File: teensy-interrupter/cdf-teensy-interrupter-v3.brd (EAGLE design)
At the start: 66 x 45.7 mm, 42 parts, among them IC1 TP4056, Q1 BC817-40LT1SMD

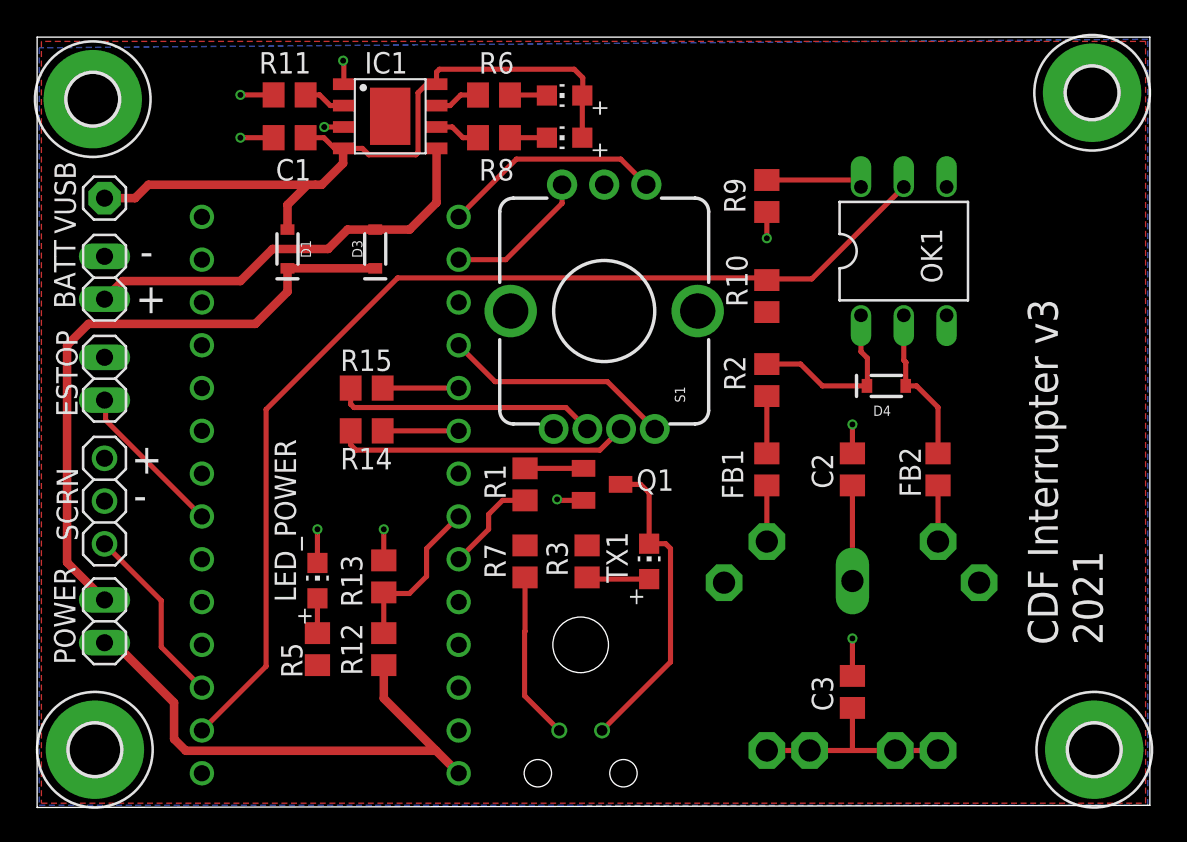
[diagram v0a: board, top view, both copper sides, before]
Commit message: V3r1
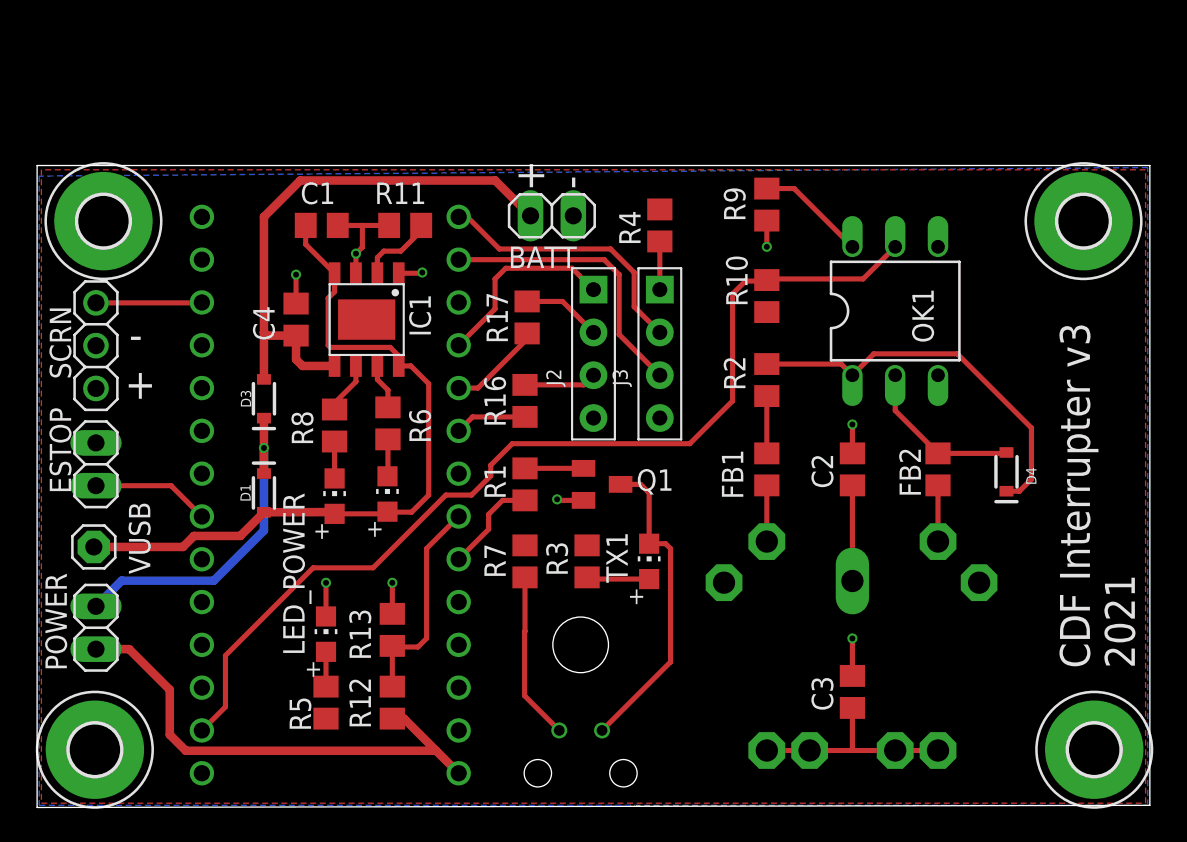
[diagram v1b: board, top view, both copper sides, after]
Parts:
- removed R14, R15: 100, rcl:R0805
- removed S1: ENCODER-2LED, SparkFun-Switches:ENCODER_LED_2
- added C4: 10uF, rcl:C0805
- added J2, J3: 4p-2.54, OPL_Connector:H4-2.54
- added R16, R17: 100, rcl:R0805
- added R4: 10k, rcl:R0805
- R11: value 1.2K -> 10k
- moved BATT 26.8 mm to (30.6, 35.1), turned to 180 degrees
- moved CHARGING 25.9 mm to (20.8, 18.6), turned to 0 degrees
- moved CHARGED 25.3 mm to (17.7, 18.5), turned to 0 degrees
- moved VUSB 20.7 mm to (3.37, 15.5)
- moved R6 20.5 mm to (20.8, 22.8), turned to 270 degrees
- moved R8 19.5 mm to (17.7, 22.7), turned to 270 degrees
- moved D1 14.5 mm to (13.5, 18.7), turned to 270 degrees
- moved IC1 12.1 mm to (19.6, 29.0), turned to 270 degrees
- moved D3 11.1 mm to (13.5, 24.3)
- moved R11 10.3 mm to (21.8, 34.5)
- moved SCRN 9.24 mm to (3.49, 27.4), turned to 270 degrees
- moved D4 8.77 mm to (57.5, 19.9), turned to 90 degrees
- moved H2 7.64 mm to (62.1, 34.8)
- moved H4 7.27 mm to (3.94, 34.8)
- moved C1 5.54 mm to (16.9, 34.5), turned to 0 degrees
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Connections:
- net N$20 renamed SW
- net N$22 renamed V_USB
- removed net N$25: R15.2, S1.+G
- removed net N$26: R14.2, S1.+R
- new net N$20: J2.3, R16.1
- new net N$5: J3.1, R4.2
- new net N$6: J2.2, R17.1
- net +3V3: now also R4.1; no longer S1.C
- net B+: now also C4.1
- net ENC_A: now also J3.2; no longer S1.A
- net ENC_B: now also J3.3; no longer S1.B
- net ENC_Z: now also J2.1; no longer S1.SW
- net GND: now also C4.2, J2.4; no longer S1.GND
- net IND_G: now also R17.2; no longer R15.1
- net IND_R: now also R16.2; no longer R14.1
- net SCRN_TX: now also TEENSY.10; no longer TEENSY.1
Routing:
- net N$26: track 17.5 -> 0.00 mm
- net SW: track 37.0 -> 20.0 mm, vias 0 -> 1
- net N$25: track 15.6 -> 0.00 mm
- net N$2: track 10.8 -> 23.1 mm
- net ENC_B: track 8.63 -> 16.9 mm
- net B+: track 25.3 -> 33.1 mm
- net MIDI_RX: track 64.1 -> 58.9 mm
- net N$6: track 0.00 -> 4.70 mm
- net SCRN_TX: track 10.9 -> 6.30 mm
- net N$20: track 0.00 -> 4.30 mm
- net V_SENSE: track 9.75 -> 12.7 mm
- net N$5: track 0.00 -> 2.86 mm
- net ENC_A: track 13.2 -> 16.0 mm
- net GND: track 17.9 -> 20.6 mm, vias 10 -> 9
- net V+: track 31.9 -> 29.5 mm
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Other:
- board size 66 x 45.7 mm -> 66 x 38.1 mm
